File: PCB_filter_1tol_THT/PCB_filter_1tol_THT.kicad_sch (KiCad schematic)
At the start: 27 parts, among them J1 Conn_01x03_Pin, J2 Conn_01x02_Pin, U1 AD620, U2 LM2902N/NOPB, U3 LF444ACN_NOPB

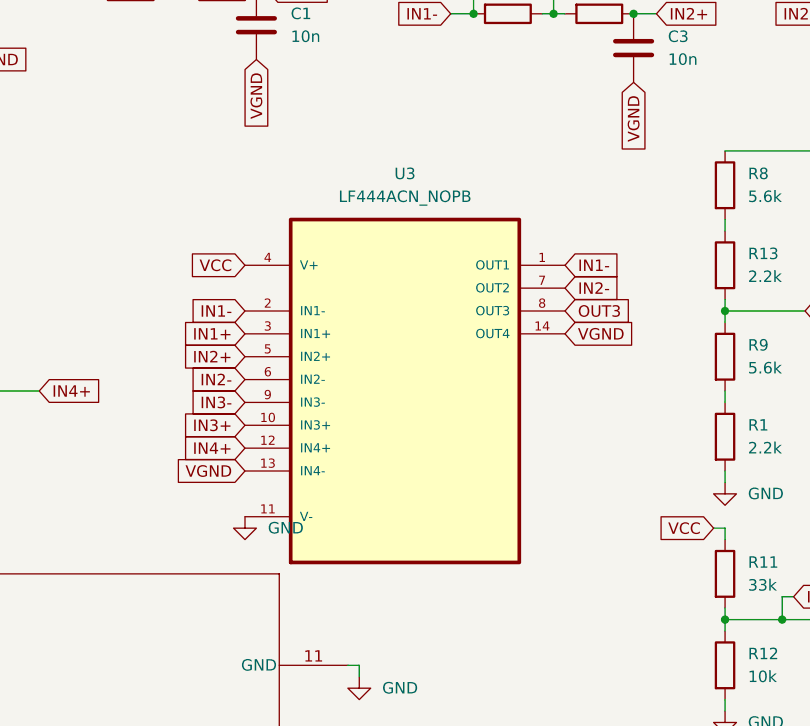
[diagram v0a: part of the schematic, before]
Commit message: last
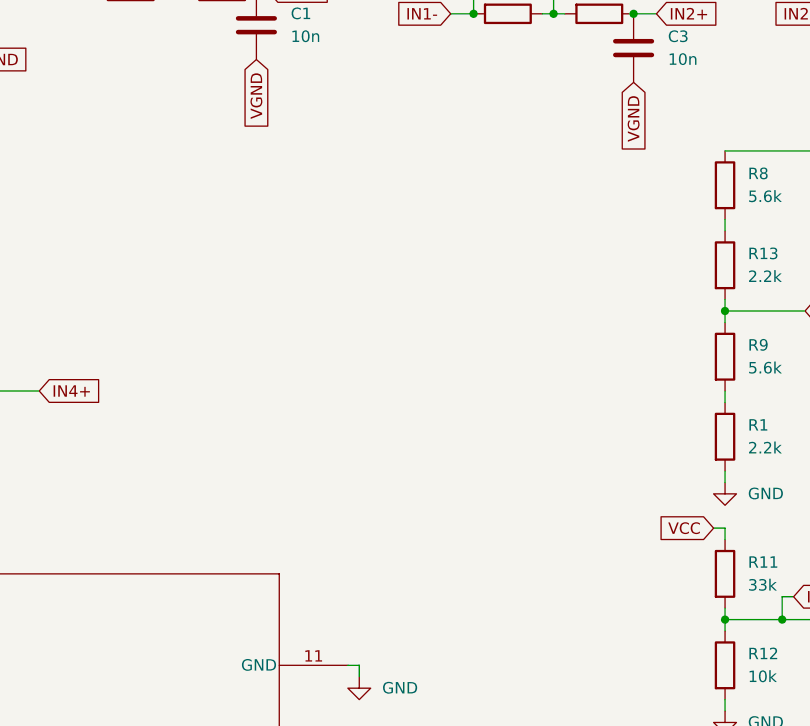
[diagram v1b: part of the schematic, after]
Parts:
- removed U3: LF444ACN_NOPB, LF444ACN_NOPB:DIP245762X508-14, symbol LF444ACN_NOPB:LF444ACN_NOPB
- R1, R10, R11, R12, R13, R14, R15, R2, R3, R4, R5, R6, R7, R8, R9: footprint Resistor_THT:R_Axial_DIN0207_L6.3mm_D2.5mm_P7.62mm_Horizontal -> DAVID:R_hueco_grande
- U2: footprint NFF_14 -> LM2902N:NFF_14
